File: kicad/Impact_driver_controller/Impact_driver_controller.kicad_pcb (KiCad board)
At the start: 2 copper layers, 208.2 x 101.1 mm, 36 parts, among them U1 DRV8874_module, U10 Control_panel_module, U2 ACS712 30A, U3 LM78M05, U4 DRV8874_module, U5 DRV8874_module, U6 MCU_module, U7 DRV8874_module, U8 DRV8874_module, U9 DRV8874_module

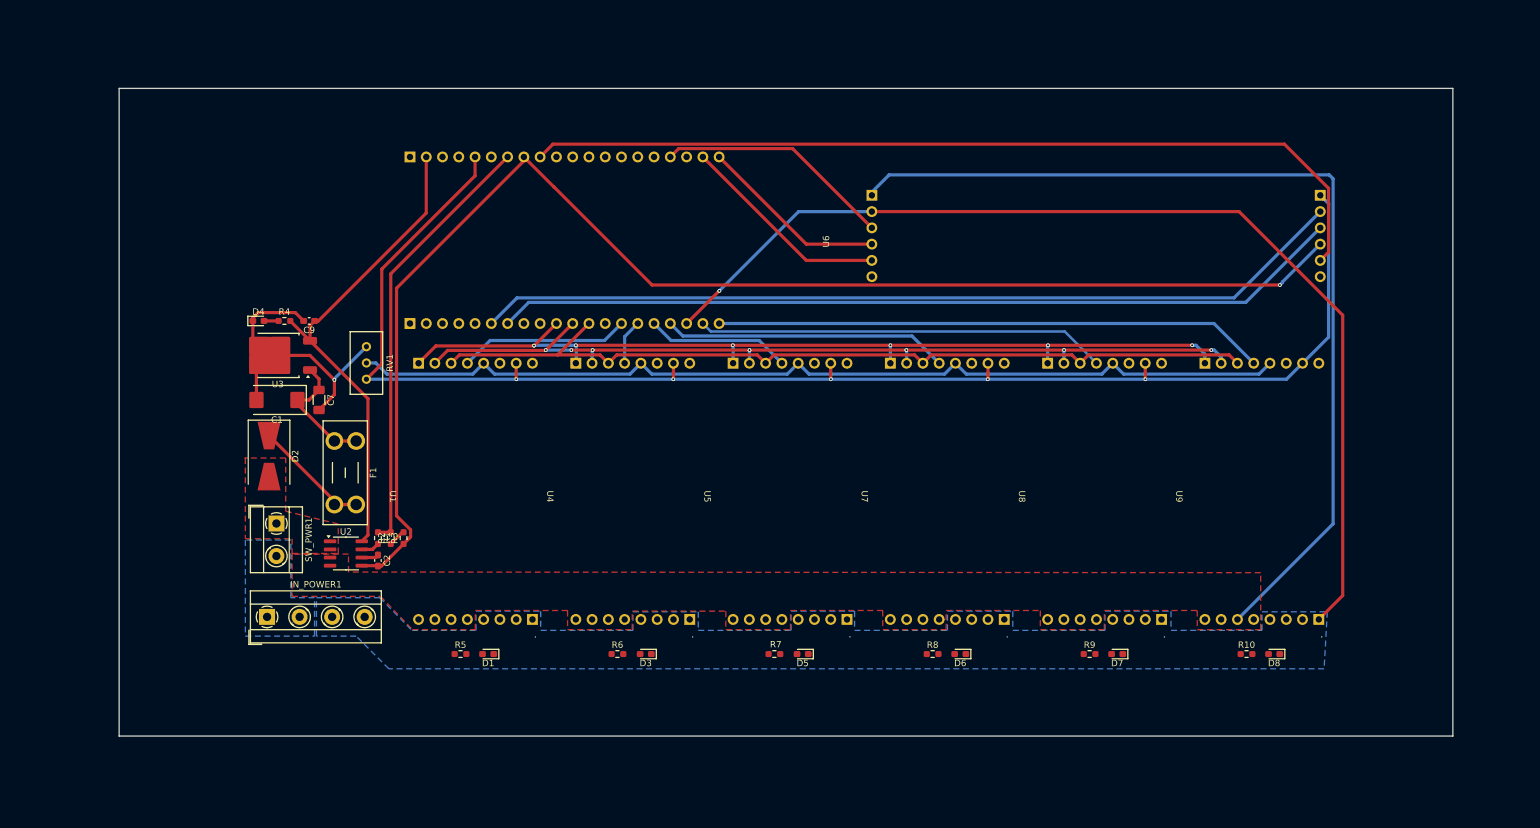
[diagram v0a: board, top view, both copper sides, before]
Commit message: main board silkscreen
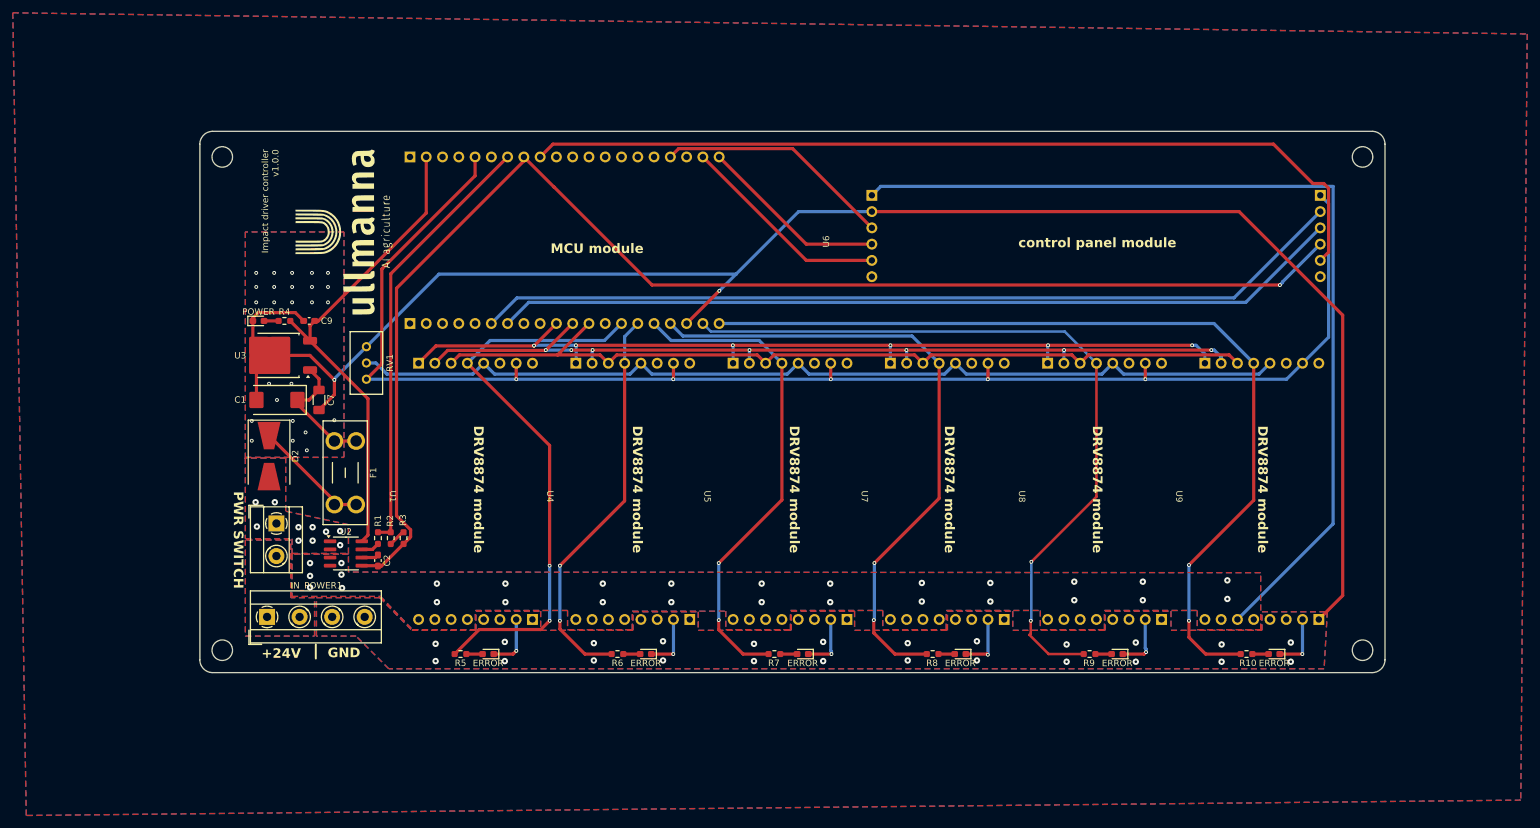
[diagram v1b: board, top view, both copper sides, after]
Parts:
- added G***: LOGO, LOGO, F.Cu at (85.0, 58.7)
- added H3: MountingHole, MountingHole:MountingHole_3.2mm_M3, F.Cu at (66.0, 47.0)
- added H3: MountingHole, MountingHole:MountingHole_3.2mm_M3, F.Cu at (244.0, 47.0)
- added H3: MountingHole, MountingHole:MountingHole_3.2mm_M3, F.Cu at (66.0, 124.0)
- added H3: MountingHole, MountingHole:MountingHole_3.2mm_M3, F.Cu at (244.0, 124.0)
- renumbered D5 to ERROR, D3 to ERROR, D6 to ERROR, D8 to ERROR, D7 to ERROR, D1 to ERROR, D4 to POWER
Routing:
- net GND: track 211.4 -> 327.1 mm, vias 2 -> 57
- net /Drivers/FAULT_1: track 26.6 -> 89.1 mm, vias 0 -> 2
- net /Drivers/FAULT_5: track 64.0 -> 120.5 mm, vias 0 -> 2
- net /Drivers/FAULT_6: track 86.0 -> 142.2 mm, vias 0 -> 2
- net /Drivers/FAULT_4: track 44.5 -> 100.5 mm, vias 0 -> 2
- net /Drivers/FAULT_2: track 7.05 -> 62.4 mm, vias 0 -> 2
- net /Drivers/FAULT_3: track 22.5 -> 77.6 mm, vias 0 -> 2
- net Net-(D5-A): track 0.00 -> 2.62 mm
- net Net-(D3-A): track 0.00 -> 2.62 mm
- net Net-(D1-A): track 0.00 -> 2.53 mm
- net Net-(D8-A): track 0.00 -> 2.52 mm
- net Net-(D7-A): track 0.00 -> 2.52 mm
- net Net-(D6-A): track 0.00 -> 2.52 mm
- net +VDD: track 148.8 -> 146.9 mm, vias 0 -> 28
- net /Current probe/IN: vias 0 -> 10
- added copper zone on B.Cu, net (none)
- added copper zone on F.Cu, net (none)
- added copper zone on B.Cu, net +VDD
- added copper zone on B.Cu, net /Current probe/IN
- added copper zone on F.Cu, net /Power supply/+V_IN
- added copper zone on F.Cu, net GND
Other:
- board size 208.2 x 101.1 mm -> 185 x 84.5 mm
- board text added: "+24V"
- board text added: "DRV8874 module"
- board text added: "GND"
- board text added: "Impact driver controller v1.0.0"
- board text added: "MCU module"
- board text added: "PWR SWITCH"
- board text added: "control panel module"
